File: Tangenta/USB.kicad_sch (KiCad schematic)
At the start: 2 parts, among them J12 907-211A1019D10200, J13 906-861A2116D10210

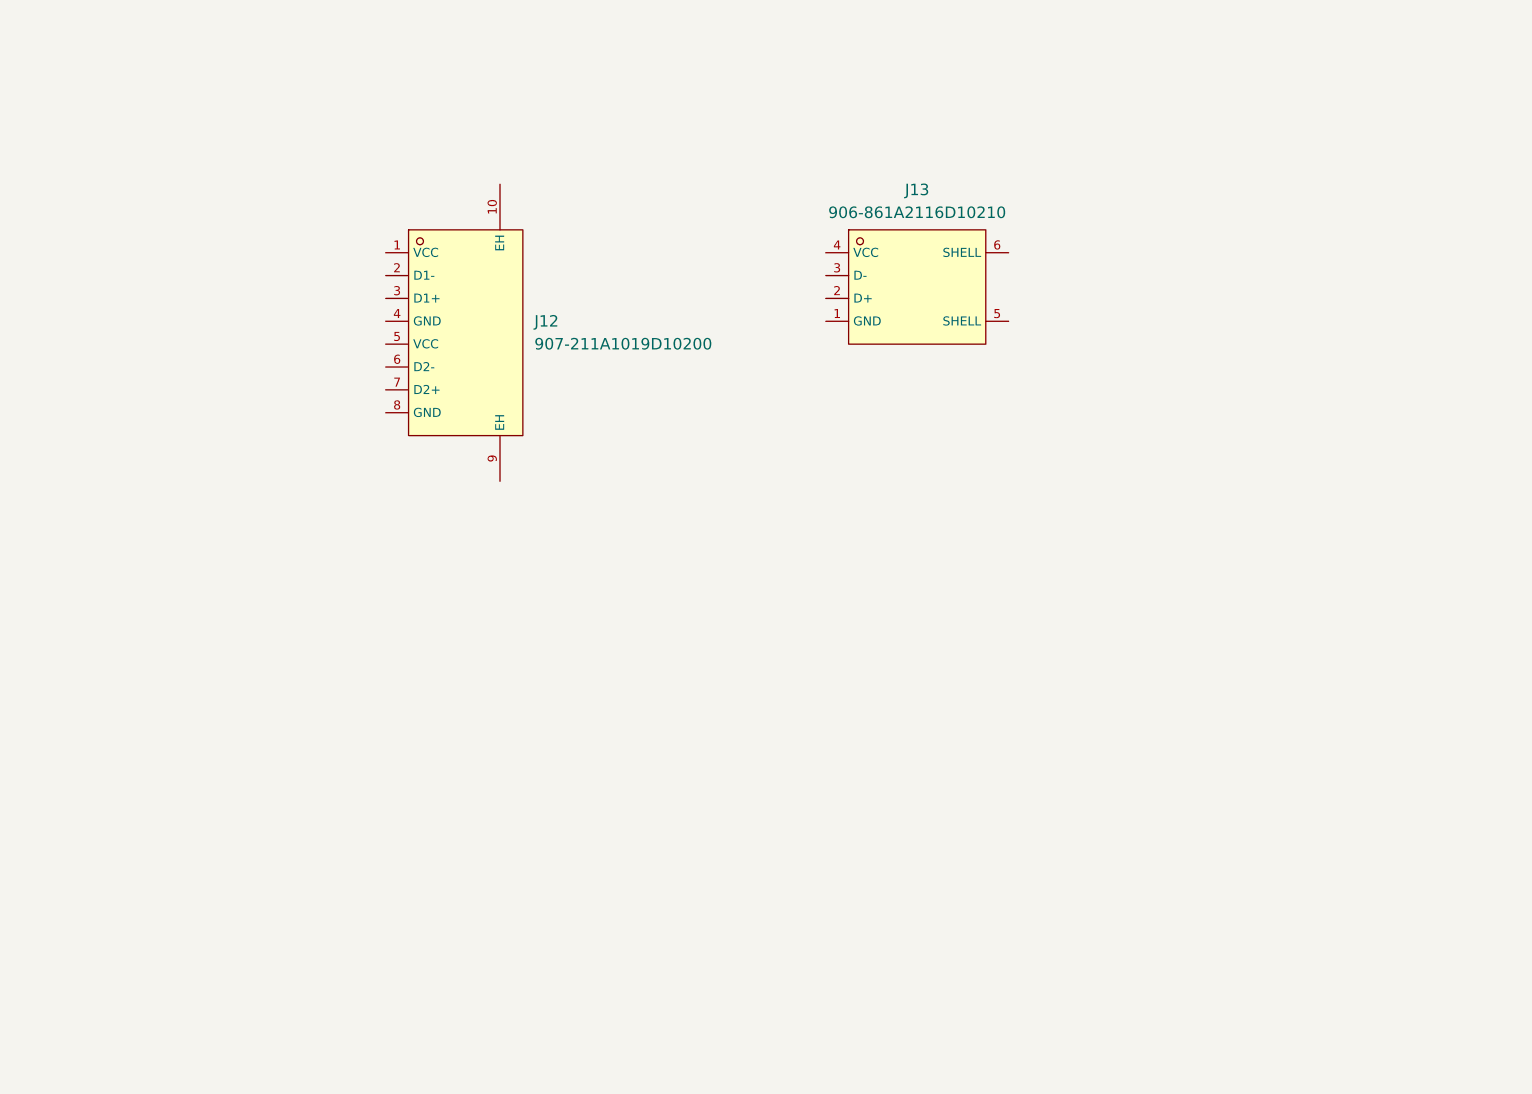
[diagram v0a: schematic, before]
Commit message: Current progress with the USB schematics...
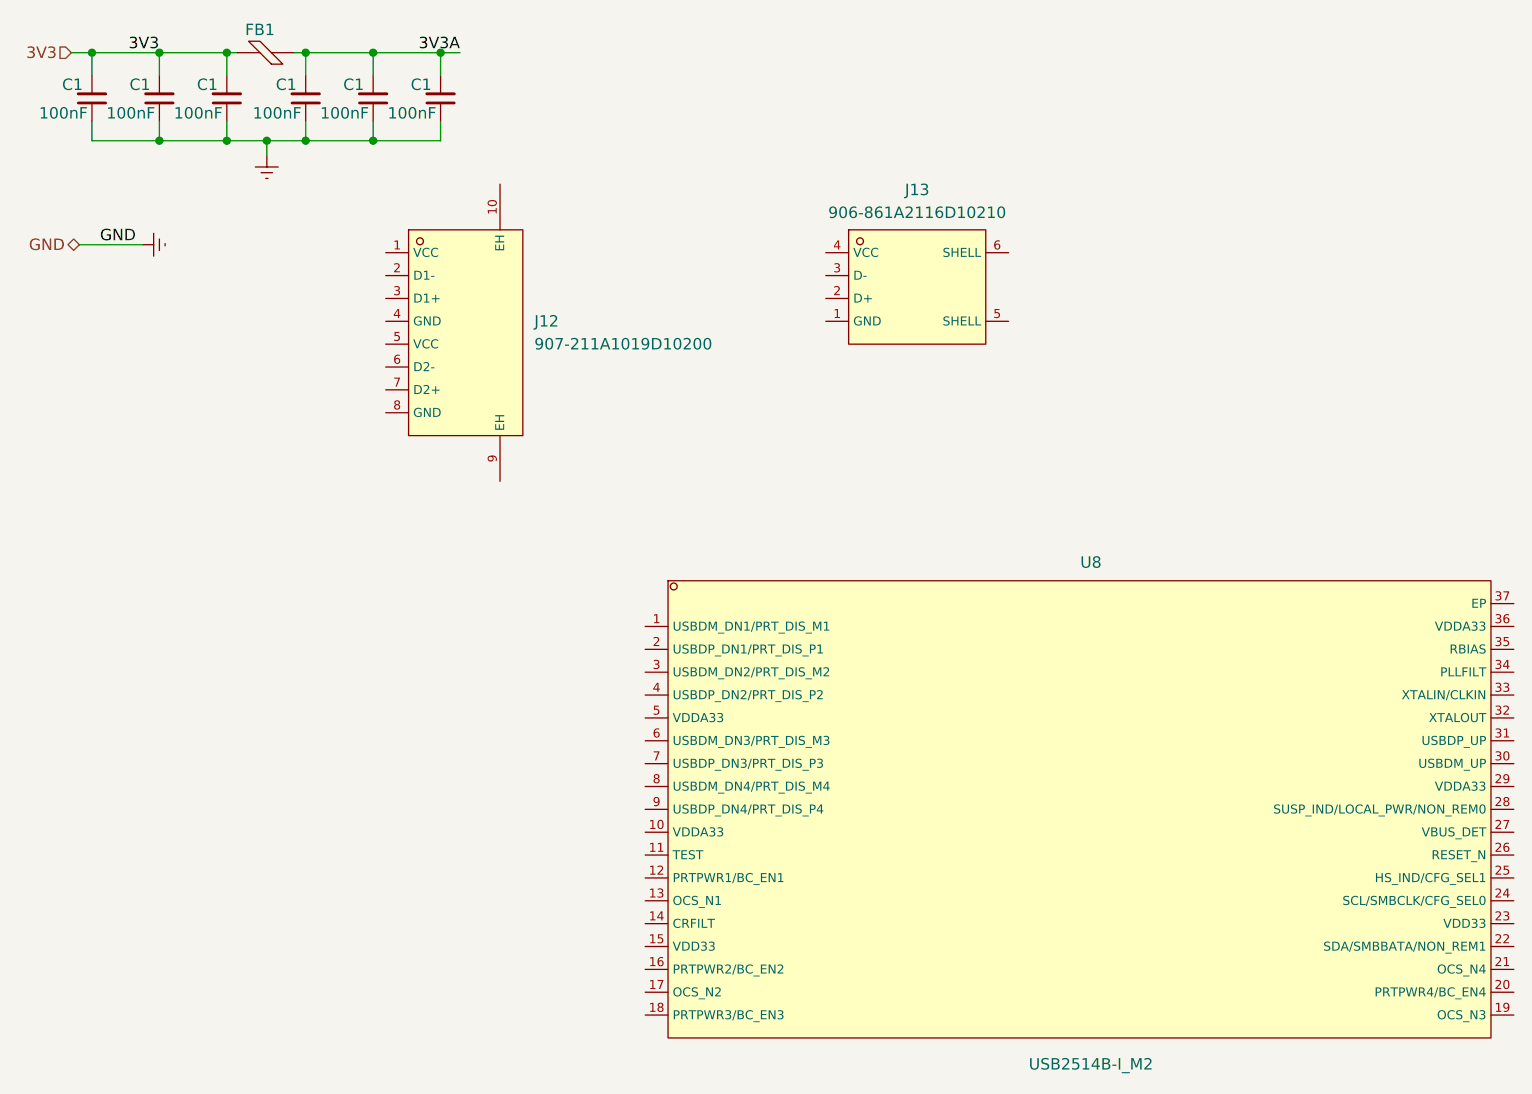
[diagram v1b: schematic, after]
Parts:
- added C1 (x6): 100nF, Capacitor_SMD:C_0402_1005Metric, symbol Device:C_Small
- added FB1: GZ2012D101TF, footprint:L0805, symbol Ferrite_Bead_100:GZ2012D101TF
- added U8: USB2514B-I_M2, USB_HUB:USB_HUB, symbol USB_HUB:USB2514B-I_M2
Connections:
- new net 3V3: C1.2, C1.2, C1.2, FB1.1
- new net 3V3A: C1.2, C1.2, C1.2, FB1.2
- new net GNDREF: C1.1, C1.1, C1.1, C1.1, C1.1, C1.1
